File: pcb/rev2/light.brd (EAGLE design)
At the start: 13 x 13 mm, 5 parts, among them J3 FFC3B07-05-T, U1 TEMT6000

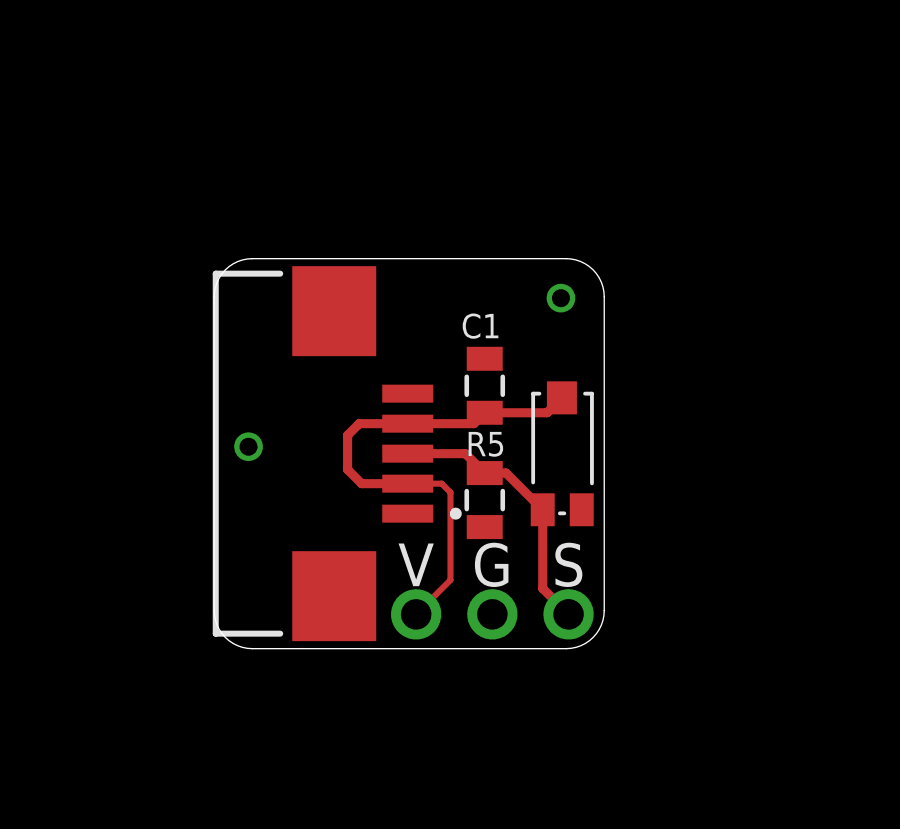
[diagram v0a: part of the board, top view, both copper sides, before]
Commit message: working on improvments
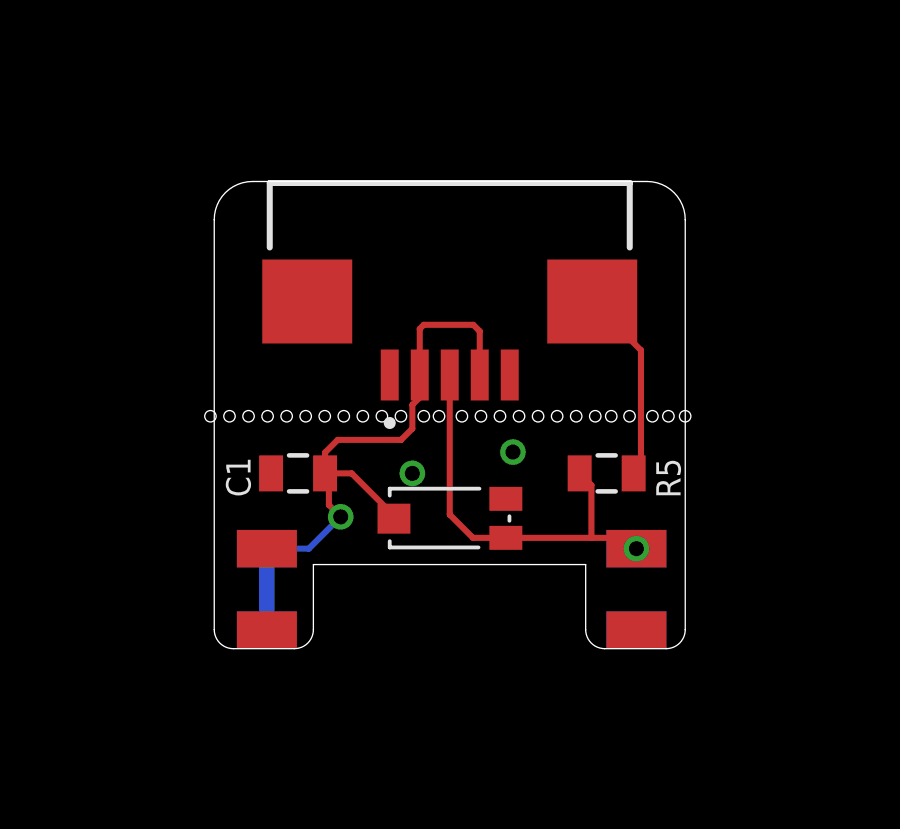
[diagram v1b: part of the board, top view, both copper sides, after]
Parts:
- removed JP1: (no value), adafruit_changed:1X03-CLEANBIG
- added U$1: LS_VERT, apricot:LS_VERT
- moved C1 6.87 mm to (2.79, 5.84), turned to 0 degrees
- moved J3 6.37 mm to (7.85, 11.6), turned to 180 degrees
- moved U1 4.33 mm to (7.85, 4.34), turned to 180 degrees
- moved R5 4.16 mm to (13.1, 5.84), turned to 180 degrees
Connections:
- net +3V3: now also U$1.B1, U$1.B2; no longer JP1.1
- net GND: now also U$1.T1, U$1.T2; no longer JP1.2
- net S: now also U$1.B3, U$1.B4, U$1.T3, U$1.T4; no longer JP1.3
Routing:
- net GND: track 0.00 -> 6.50 mm
- net S: track 9.12 -> 13.7 mm, vias 0 -> 1
- net +3V3: track 17.1 -> 21.2 mm, vias 0 -> 1
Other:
- board size 13 x 13 mm -> 15.7 x 15.6 mm
- board text added: "PulseHPT.com"
- board text removed: "G"
- board text removed: "PulseHPT.com dekuNukem 2023"
- board text removed: "S"
- board text removed: "V"
